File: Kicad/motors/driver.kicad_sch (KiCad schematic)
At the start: 38 parts

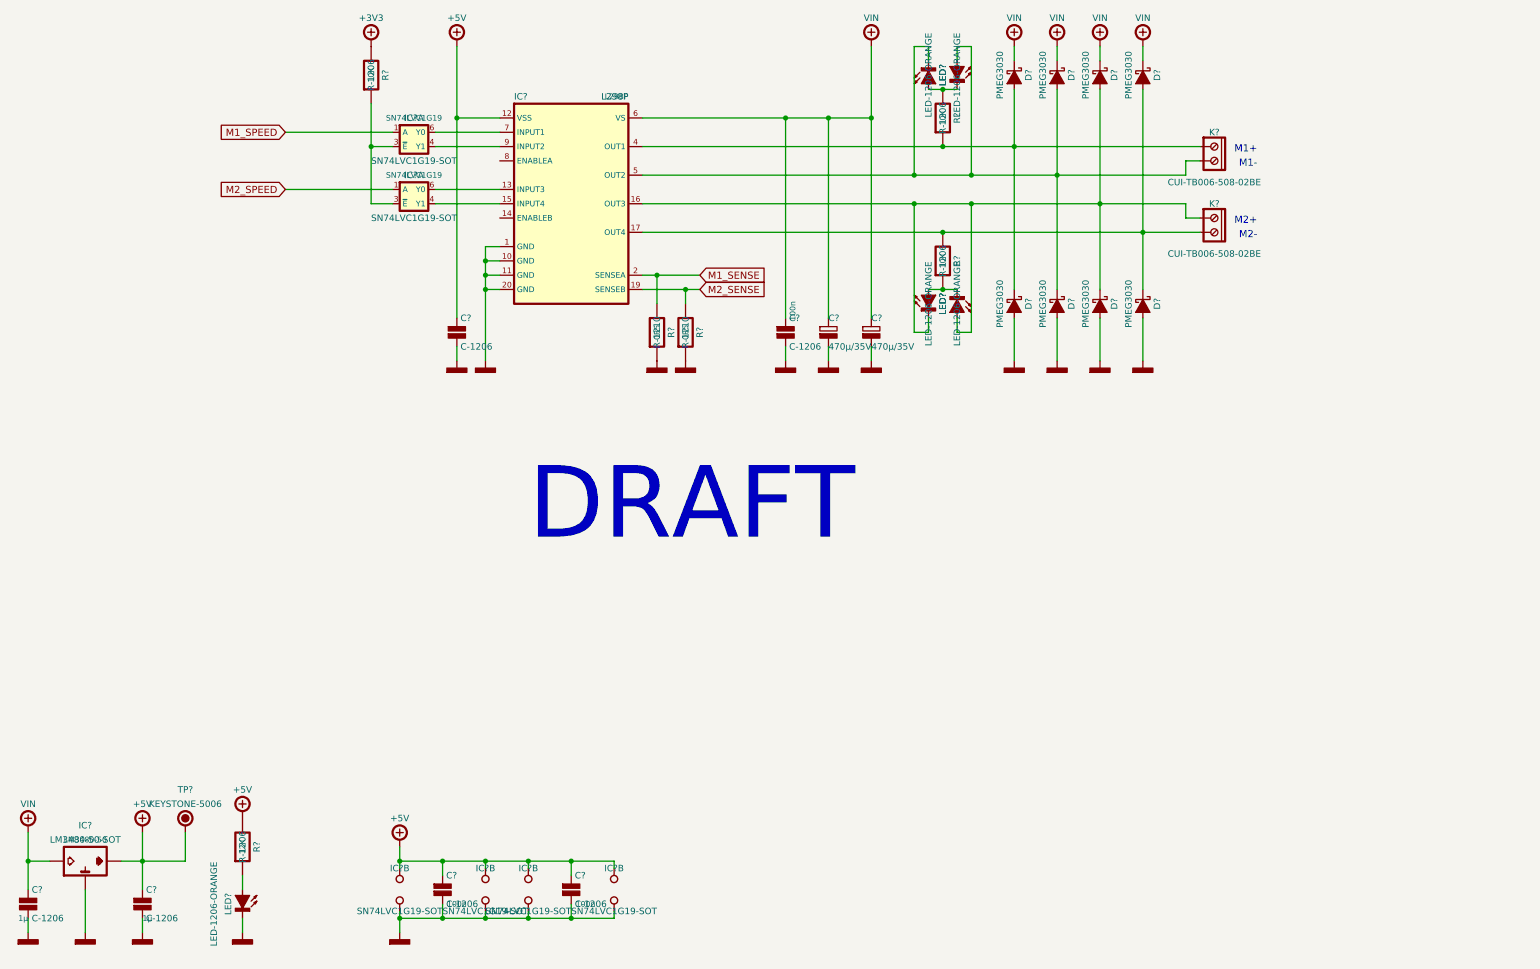
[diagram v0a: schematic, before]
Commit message: Update Motor
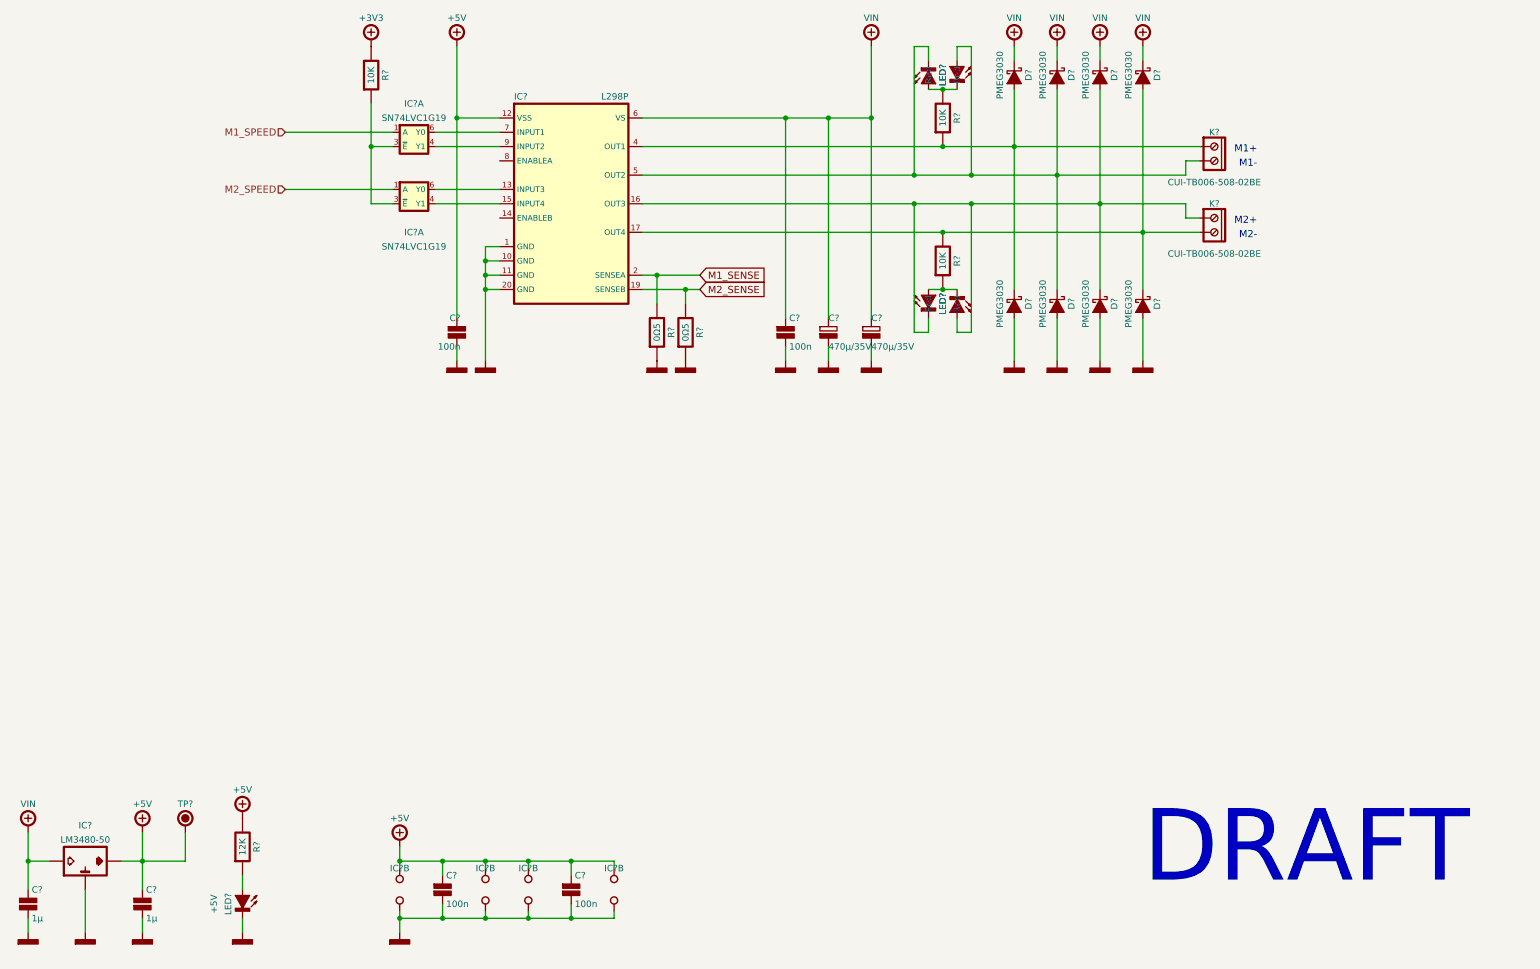
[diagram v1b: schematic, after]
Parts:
- removed TP?: KEYSTONE-5006, tronixio:KEYSTONE-5006, symbol tronixio:KEYSTONE-5006
- added TP?: HARWIN-S1751, tronixio:zzzHARWIN-S1751, symbol tronixio:HARWIN-S1751
- C?: value C-1206 -> 100n
- C? (x2): value C-1206 -> 1µ; Name 1µ -> (none)
- C? (x3): value C-1206 -> 100n; Name 100n -> (none)
- IC? (x2): value SN74LVC1G19-SOT -> SN74LVC1G19; Name SN74LVC1G19 -> (none)
- IC? (x4): Name SN74LVC1G19 -> (none)
- IC?: value LM3480-50-SOT -> LM3480-50; Name LM3480-50 -> (none)
- IC?: Name L298P -> (none)
- LED? (x4): value LED-1206-ORANGE -> Red; symbol tronixio:LED-1206-ORANGE -> tronixio:LED-1206-RED; MOUSER 604-APT3216LSECKJ4RV -> 604-APT3216LSECKJ3RV
- LED?: value LED-1206-ORANGE -> +5V; symbol tronixio:LED-1206-ORANGE -> tronixio:LED-1206-RED; MOUSER 604-APT3216LSECKJ4RV -> 604-APT3216LSECKJ3RV
- R? (x3): value R-1206 -> 10K; Name 10K -> (none)
- R? (x2): value R-1210 -> 0Ω5; Name 0R5 -> (none)
- R?: value R-1206 -> 12K; Name 12K -> (none)
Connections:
- net +5V: now also TP?.1
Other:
- title: Motor Driver -> Motors Driver
